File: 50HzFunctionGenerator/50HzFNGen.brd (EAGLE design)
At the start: 99 x 77.1 mm, 32 parts, among them IC1 LM311N, IC2 7812L, IC4 TL082P, X2 MAB32

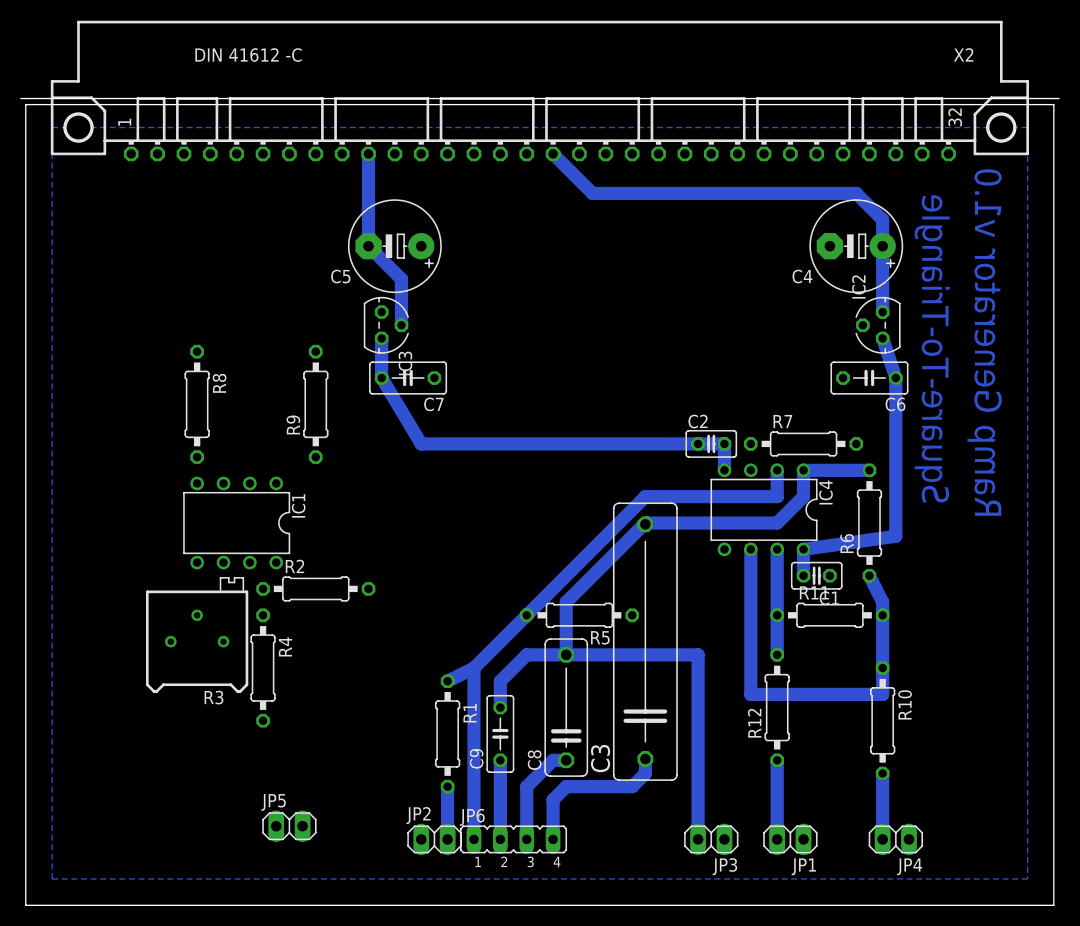
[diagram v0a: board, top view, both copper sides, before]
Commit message: finished version of the board
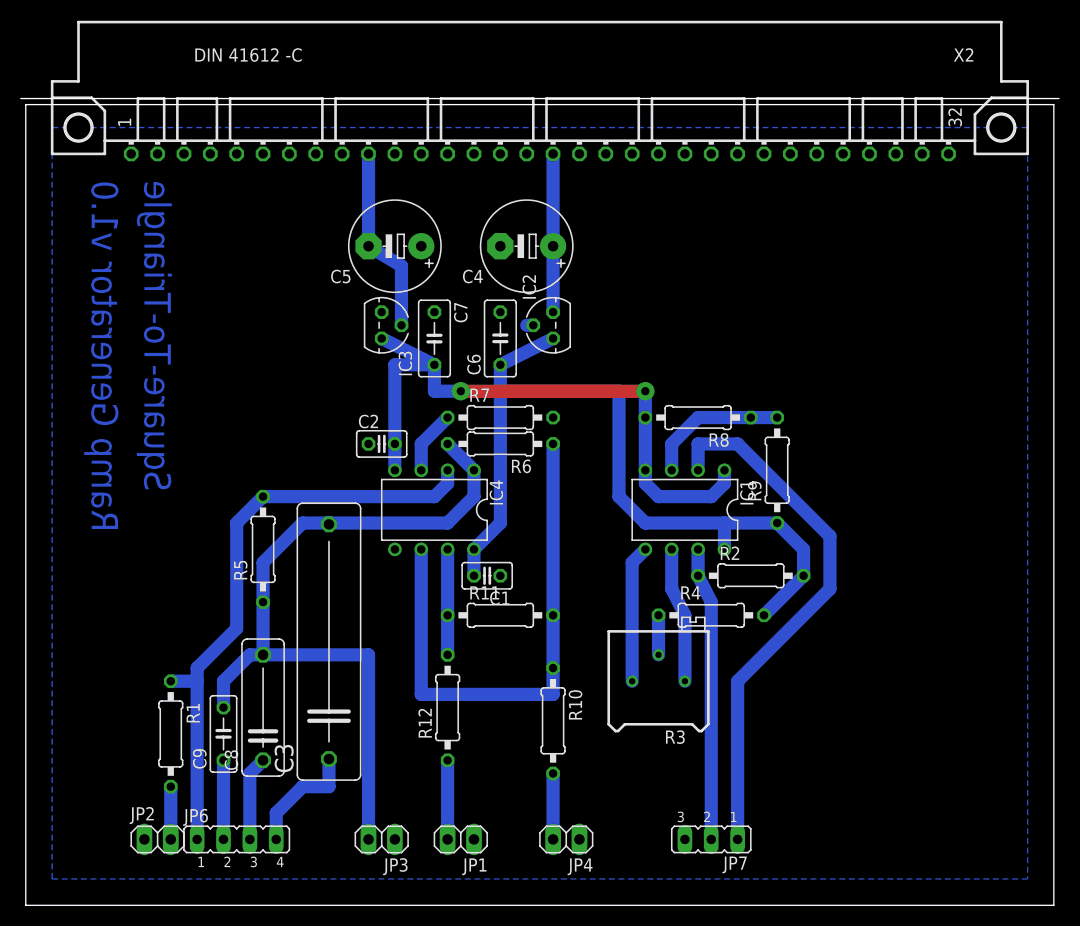
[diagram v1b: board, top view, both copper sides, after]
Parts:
- removed JP5: 5V Hz Square wave in, pinhead:1X02
- added JP7: (no value), jumper:JP2
- moved R8 48.3 mm to (64.8, 47.0), turned to 180 degrees
- moved R9 44.9 mm to (72.4, 41.9)
- moved R3 44.6 mm to (61.0, 21.6)
- moved R4 43.5 mm to (66.0, 27.9), turned to 0 degrees
- moved IC1 43.2 mm to (63.5, 38.1)
- moved R2 41.9 mm to (69.8, 31.8)
- moved R6 36.4 mm to (45.7, 44.5), turned to 180 degrees
- moved C6 35.8 mm to (45.7, 54.6), turned to 90 degrees
- moved C2 31.8 mm to (34.3, 44.5)
- moved C4 31.8 mm to (48.3, 63.5)
- moved IC4 31.8 mm to (39.4, 38.1)
- moved JP3 31.8 mm to (34.3, 6.35)
- moved C1 31.8 mm to (44.5, 31.8)
- moved IC2 31.8 mm to (50.8, 55.9)
- moved JP1 31.8 mm to (41.9, 6.35)
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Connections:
- net GND: now also JP7.3, X2.A11, X2.A12, X2.A14, X2.A15, X2.A16; no longer JP5.1
- net N$12: now also JP7.2; no longer JP2.1
- net N$23: now also JP7.1; no longer JP5.2
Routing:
- net N$23: track 0.00 -> 51.8 mm
- net +12V: track 30.8 -> 79.0 mm
- net N$12: track 0.00 -> 28.2 mm
- net +15V: track 43.3 -> 15.2 mm
- net -12V: track 43.0 -> 61.3 mm, vias 0 -> 6
- net N$25: track 0.00 -> 13.8 mm
- net N$16: track 0.00 -> 13.2 mm
- net N$18: track 0.00 -> 13.0 mm
- net N$7: track 38.4 -> 50.8 mm
- net N$14: track 81.5 -> 73.4 mm
- net N$20: track 0.00 -> 6.13 mm
- net N$19: track 0.00 -> 3.81 mm
- net N$4: track 15.1 -> 11.3 mm
- net N$11: track 9.94 -> 8.15 mm
- net GND: track 0.00 -> 0.64 mm
